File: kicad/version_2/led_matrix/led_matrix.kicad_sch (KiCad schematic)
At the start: 36 parts

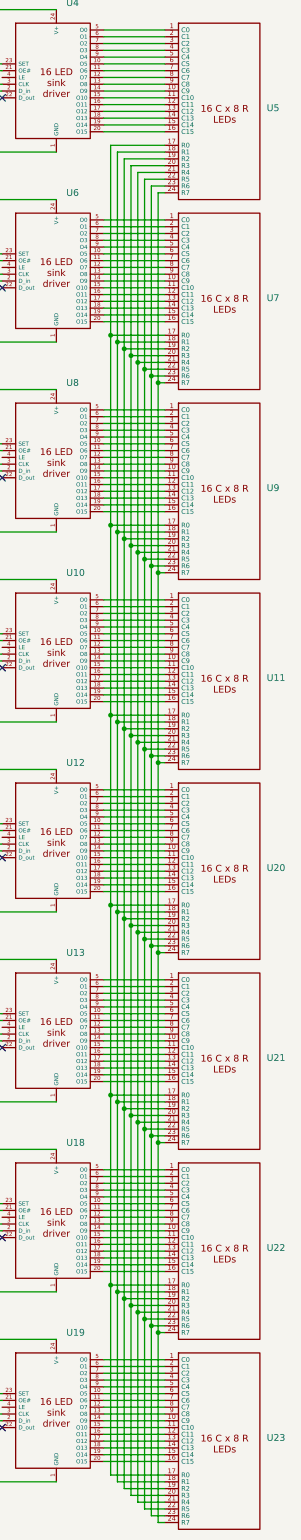
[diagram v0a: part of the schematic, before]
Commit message: Sick new LED block footprints
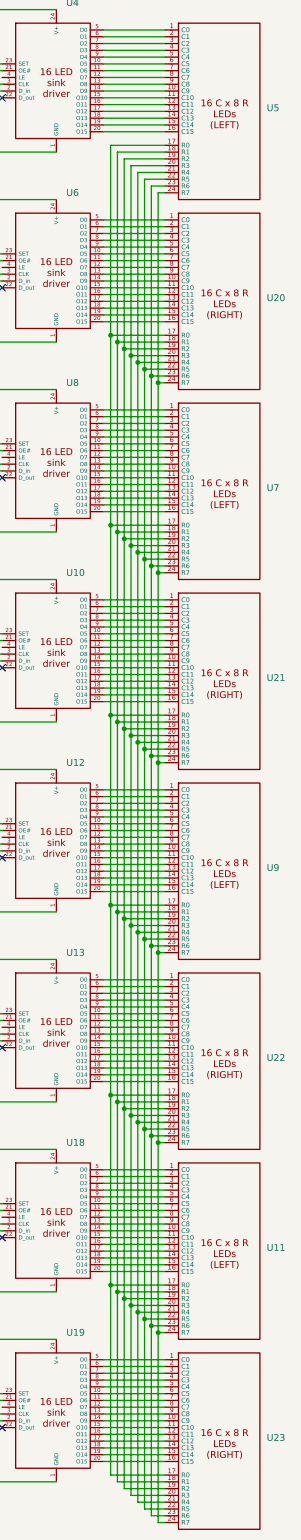
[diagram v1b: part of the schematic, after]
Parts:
- removed U11, U20, U21, U22, U23, U5, U7, U9: ~, custom_footprint_library:led_block_16_x_8, symbol custom_symbol_lib:led_block_16_x_8
- added U11, U5, U7, U9: ~, custom_footprint_library:led_block_16_x_8_left, symbol custom_symbol_lib:led_block_16_x_8_left
- added U20, U21, U22, U23: ~, custom_footprint_library:led_block_16_x_8_right, symbol custom_symbol_lib:led_block_16_x_8_right
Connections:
- net at U8.5 (O0): now also U7.1 (C0)
- net at U8.14 (O9): now also U7.10 (C9)
- net at U8.15 (O10): now also U7.11 (C10)
- net at U8.16 (O11): now also U7.12 (C11)
- net at U8.17 (O12): now also U7.13 (C12)
- net at U8.18 (O13): now also U7.14 (C13)
- net at U8.19 (O14): now also U7.15 (C14)
- net at U8.20 (O15): now also U7.16 (C15)
- net at U8.6 (O1): now also U7.2 (C1)
- net at U8.7 (O2): now also U7.3 (C2)
- net at U8.8 (O3): now also U7.4 (C3)
- net at U8.9 (O4): now also U7.5 (C4)
- net at U8.10 (O5): now also U7.6 (C5)
- net at U8.11 (O6): now also U7.7 (C6)
- net at U8.12 (O7): now also U7.8 (C7)
- net at U8.13 (O8): now also U7.9 (C8)
- net at U13.10 (O5): now also U22.6 (C5)
- net at U13.11 (O6): now also U22.7 (C6)
- net at U13.12 (O7): now also U22.8 (C7)
- net at U13.13 (O8): now also U22.9 (C8)
- net at U13.14 (O9): now also U22.10 (C9)
- net at U13.15 (O10): now also U22.11 (C10)
- net at U13.16 (O11): now also U22.12 (C11)
- net at U13.17 (O12): now also U22.13 (C12)
- net at U13.18 (O13): now also U22.14 (C13)
- net at U13.19 (O14): now also U22.15 (C14)
- net at U13.20 (O15): now also U22.16 (C15)
- net at U13.5 (O0): now also U22.1 (C0)
- net at U13.6 (O1): now also U22.2 (C1)
- net at U13.7 (O2): now also U22.3 (C2)
- net at U13.8 (O3): now also U22.4 (C3)
- net at U13.9 (O4): now also U22.5 (C4)
- net at U12.10 (O5): now also U9.6 (C5)
- net at U12.11 (O6): now also U9.7 (C6)
- net at U12.12 (O7): now also U9.8 (C7)
- net at U12.13 (O8): now also U9.9 (C8)
- net at U12.14 (O9): now also U9.10 (C9)
- net at U12.15 (O10): now also U9.11 (C10)
- net at U12.16 (O11): now also U9.12 (C11)
- net at U12.17 (O12): now also U9.13 (C12)
- net at U12.18 (O13): now also U9.14 (C13)
- net at U12.19 (O14): now also U9.15 (C14)
- net at U12.20 (O15): now also U9.16 (C15)
- net at U12.5 (O0): now also U9.1 (C0)
- net at U12.6 (O1): now also U9.2 (C1)
- net at U12.7 (O2): now also U9.3 (C2)
- net at U12.8 (O3): now also U9.4 (C3)
- net at U12.9 (O4): now also U9.5 (C4)
- net at U6.5 (O0): now also U20.1 (C0)
- net at U6.14 (O9): now also U20.10 (C9)
- net at U6.15 (O10): now also U20.11 (C10)
- net at U6.16 (O11): now also U20.12 (C11)
- net at U6.17 (O12): now also U20.13 (C12)
- net at U6.18 (O13): now also U20.14 (C13)
- net at U6.19 (O14): now also U20.15 (C14)
- net at U6.20 (O15): now also U20.16 (C15)
- net at U6.6 (O1): now also U20.2 (C1)
- net at U6.7 (O2): now also U20.3 (C2)
- net at U6.8 (O3): now also U20.4 (C3)
- net at U6.9 (O4): now also U20.5 (C4)
- net at U6.10 (O5): now also U20.6 (C5)
- net at U6.11 (O6): now also U20.7 (C6)
- net at U6.12 (O7): now also U20.8 (C7)
- net at U6.13 (O8): now also U20.9 (C8)
- net at U4.5 (O0): now also U5.1 (C0)
- net at U4.14 (O9): now also U5.10 (C9)
- net at U4.15 (O10): now also U5.11 (C10)
- net at U4.16 (O11): now also U5.12 (C11)
- net at U4.17 (O12): now also U5.13 (C12)
- net at U4.18 (O13): now also U5.14 (C13)
- net at U4.19 (O14): now also U5.15 (C14)
- net at U4.20 (O15): now also U5.16 (C15)
- net at U4.6 (O1): now also U5.2 (C1)
- net at U4.7 (O2): now also U5.3 (C2)
- net at U4.8 (O3): now also U5.4 (C3)
- net at U4.9 (O4): now also U5.5 (C4)
- net at U4.10 (O5): now also U5.6 (C5)
- net at U4.11 (O6): now also U5.7 (C6)
- net at U4.12 (O7): now also U5.8 (C7)
- net at U4.13 (O8): now also U5.9 (C8)
- net at U10.10 (O5): now also U21.6 (C5)
- net at U10.11 (O6): now also U21.7 (C6)
- net at U10.12 (O7): now also U21.8 (C7)
- net at U10.13 (O8): now also U21.9 (C8)
- net at U10.14 (O9): now also U21.10 (C9)
- net at U10.15 (O10): now also U21.11 (C10)
- net at U10.16 (O11): now also U21.12 (C11)
- net at U10.17 (O12): now also U21.13 (C12)
- net at U10.18 (O13): now also U21.14 (C13)
- net at U10.19 (O14): now also U21.15 (C14)
- net at U10.20 (O15): now also U21.16 (C15)
- net at U10.5 (O0): now also U21.1 (C0)
- net at U10.6 (O1): now also U21.2 (C1)
- net at U10.7 (O2): now also U21.3 (C2)
- net at U10.8 (O3): now also U21.4 (C3)
- net at U10.9 (O4): now also U21.5 (C4)
- net at U18.5 (O0): now also U11.1 (C0)
- net at U18.14 (O9): now also U11.10 (C9)
- net at U18.15 (O10): now also U11.11 (C10)
- net at U18.16 (O11): now also U11.12 (C11)
- net at U18.17 (O12): now also U11.13 (C12)
- net at U18.18 (O13): now also U11.14 (C13)
- net at U18.19 (O14): now also U11.15 (C14)
- net at U18.20 (O15): now also U11.16 (C15)
- net at U18.6 (O1): now also U11.2 (C1)
- net at U18.7 (O2): now also U11.3 (C2)
- net at U18.8 (O3): now also U11.4 (C3)
- net at U18.9 (O4): now also U11.5 (C4)
- net at U18.10 (O5): now also U11.6 (C5)
- net at U18.11 (O6): now also U11.7 (C6)
- net at U18.12 (O7): now also U11.8 (C7)
- net at U18.13 (O8): now also U11.9 (C8)
- net at U19.10 (O5): now also U23.6 (C5)
- net at U19.11 (O6): now also U23.7 (C6)
- net at U19.12 (O7): now also U23.8 (C7)
- net at U19.13 (O8): now also U23.9 (C8)
- net at U19.14 (O9): now also U23.10 (C9)
- net at U19.15 (O10): now also U23.11 (C10)
- net at U19.16 (O11): now also U23.12 (C11)
- net at U19.17 (O12): now also U23.13 (C12)
- net at U19.18 (O13): now also U23.14 (C13)
- net at U19.19 (O14): now also U23.15 (C14)
- net at U19.20 (O15): now also U23.16 (C15)
- net at U19.5 (O0): now also U23.1 (C0)
- net at U19.6 (O1): now also U23.2 (C1)
- net at U19.7 (O2): now also U23.3 (C2)
- net at U19.8 (O3): now also U23.4 (C3)
- net at U19.9 (O4): now also U23.5 (C4)
- new net: U11.17 (R0), U20.17 (R0), U21.17 (R0), U22.17 (R0), U23.17 (R0), U5.17 (R0), U7.17 (R0), U9.17 (R0)
- new net: U11.18 (R1), U20.18 (R1), U21.18 (R1), U22.18 (R1), U23.18 (R1), U5.18 (R1), U7.18 (R1), U9.18 (R1)
- new net: U11.19 (R2), U20.19 (R2), U21.19 (R2), U22.19 (R2), U23.19 (R2), U5.19 (R2), U7.19 (R2), U9.19 (R2)
- new net: U11.20 (R3), U20.20 (R3), U21.20 (R3), U22.20 (R3), U23.20 (R3), U5.20 (R3), U7.20 (R3), U9.20 (R3)
- new net: U11.21 (R4), U20.21 (R4), U21.21 (R4), U22.21 (R4), U23.21 (R4), U5.21 (R4), U7.21 (R4), U9.21 (R4)
- new net: U11.22 (R5), U20.22 (R5), U21.22 (R5), U22.22 (R5), U23.22 (R5), U5.22 (R5), U7.22 (R5), U9.22 (R5)
- new net: U11.23 (R6), U20.23 (R6), U21.23 (R6), U22.23 (R6), U23.23 (R6), U5.23 (R6), U7.23 (R6), U9.23 (R6)
- new net: U11.24 (R7), U20.24 (R7), U21.24 (R7), U22.24 (R7), U23.24 (R7), U5.24 (R7), U7.24 (R7), U9.24 (R7)
